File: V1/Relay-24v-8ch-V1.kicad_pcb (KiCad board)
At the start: 2 copper layers, 108 x 67.8 mm, 49 parts, among them J1 Conn_01x09, J2 OUT1, J3 OUT2, J4 OUT3, J5 OUT4, J6 OUT5, J7 OUT6, J8 OUT7, J9 OUT8, K1 G5PZ-1A, K2 G5PZ-1A, K3 G5PZ-1A, K4 G5PZ-1A, K5 G5PZ-1A, K6 G5PZ-1A, K7 G5PZ-1A, K8 G5PZ-1A

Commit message: Adjustments for fabrication
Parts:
- D11, D12, D15, D16, D3, D4, D7, D8: value BLUE/0603 -> GREEN/0603
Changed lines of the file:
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@@
     (property "Case" "0603")
     (property "JLCPCB BOM" "1")
-    (property "LCSC Part #" "C72041")
+    (property "LCSC Part #" "C72043")
     (property "Mfr" "Everlight")
-    (property "Mfr PN" "19-217/BHC-ZL1M2RY/3T")
+    (property "Mfr PN" "19-217/GHC-YR1S2/3T")
     (property "Sheetfile" "Relay-24v-8ch-V1.kicad_sch")
     (property "Sheetname" "")
     (property "Technology" "")
     (property "Vendor" "JLCPCB")
-    (property "Vendor PN" "C72041")
+    (property "Vendor PN" "C72043")
     (property "ki_description" "Light emitting diode")
     (property "ki_keywords" "LED diode")
@@
         (effects (font (size 1 1) (thickness 0.15)))
     )
-    (fp_text value "BLUE/0603" (at 0 1.43) (layer "F.Fab")
+    (fp_text value "GREEN/0603" (at 0 1.43) (layer "F.Fab")
         (effects (font (size 1 1) (thickness 0.15)))
     )
@@
     (property "Case" "0603")
     (property "JLCPCB BOM" "1")
-    (property "LCSC Part #" "C72041")
+    (property "LCSC Part #" "C72043")
     (property "Mfr" "Everlight")
-    (property "Mfr PN" "19-217/BHC-ZL1M2RY/3T")
+    (property "Mfr PN" "19-217/GHC-YR1S2/3T")
     (property "Sheetfile" "Relay-24v-8ch-V1.kicad_sch")
     (property "Sheetname" "")
     (property "Technology" "")
     (property "Vendor" "JLCPCB")
-    (property "Vendor PN" "C72041")
+    (property "Vendor PN" "C72043")
     (property "ki_description" "Light emitting diode")
     (property "ki_keywords" "LED diode")
@@
         (effects (font (size 1 1) (thickness 0.15)))
     )
-    (fp_text value "BLUE/0603" (at 0 1.43) (layer "F.Fab")
+    (fp_text value "GREEN/0603" (at 0 1.43) (layer "F.Fab")
         (effects (font (size 1 1) (thickness 0.15)))
     )
@@
     (property "Case" "0603")
     (property "JLCPCB BOM" "1")
-    (property "LCSC Part #" "C72041")
+    (property "LCSC Part #" "C72043")
     (property "Mfr" "Everlight")
-    (property "Mfr PN" "19-217/BHC-ZL1M2RY/3T")
+    (property "Mfr PN" "19-217/GHC-YR1S2/3T")
     (property "Sheetfile" "Relay-24v-8ch-V1.kicad_sch")
     (property "Sheetname" "")
     (property "Technology" "")
     (property "Vendor" "JLCPCB")
-    (property "Vendor PN" "C72041")
+    (property "Vendor PN" "C72043")
     (property "ki_description" "Light emitting diode")
     (property "ki_keywords" "LED diode")
@@
         (effects (font (size 1 1) (thickness 0.15)))
     )
-    (fp_text value "BLUE/0603" (at 0 1.43) (layer "F.Fab")
+    (fp_text value "GREEN/0603" (at 0 1.43) (layer "F.Fab")
         (effects (font (size 1 1) (thickness 0.15)))
     )
@@
     (property "Case" "0603")
     (property "JLCPCB BOM" "1")
-    (property "LCSC Part #" "C72041")
+    (property "LCSC Part #" "C72043")
     (property "Mfr" "Everlight")
-    (property "Mfr PN" "19-217/BHC-ZL1M2RY/3T")
+    (property "Mfr PN" "19-217/GHC-YR1S2/3T")
     (property "Sheetfile" "Relay-24v-8ch-V1.kicad_sch")
     (property "Sheetname" "")
     (property "Technology" "")
     (property "Vendor" "JLCPCB")
-    (property "Vendor PN" "C72041")
+    (property "Vendor PN" "C72043")
     (property "ki_description" "Light emitting diode")
     (property "ki_keywords" "LED diode")
@@
         (effects (font (size 1 1) (thickness 0.15)))
     )
-    (fp_text value "BLUE/0603" (at 0 1.43) (layer "F.Fab")
+    (fp_text value "GREEN/0603" (at 0 1.43) (layer "F.Fab")
         (effects (font (size 1 1) (thickness 0.15)))
     )
@@
     (property "Case" "0603")
     (property "JLCPCB BOM" "1")
-    (property "LCSC Part #" "C72041")
+    (property "LCSC Part #" "C72043")
     (property "Mfr" "Everlight")
-    (property "Mfr PN" "19-217/BHC-ZL1M2RY/3T")
+    (property "Mfr PN" "19-217/GHC-YR1S2/3T")
     (property "Sheetfile" "Relay-24v-8ch-V1.kicad_sch")
     (property "Sheetname" "")
     (property "Technology" "")
     (property "Vendor" "JLCPCB")
-    (property "Vendor PN" "C72041")
+    (property "Vendor PN" "C72043")
     (property "ki_description" "Light emitting diode")
     (property "ki_keywords" "LED diode")
@@
         (effects (font (size 1 1) (thickness 0.15)))
     )
-    (fp_text value "BLUE/0603" (at 0 1.43) (layer "F.Fab")
+    (fp_text value "GREEN/0603" (at 0 1.43) (layer "F.Fab")
         (effects (font (size 1 1) (thickness 0.15)))
     )
@@
     (property "Case" "0603")
     (property "JLCPCB BOM" "1")
-    (property "LCSC Part #" "C72041")
+    (property "LCSC Part #" "C72043")
     (property "Mfr" "Everlight")
-    (property "Mfr PN" "19-217/BHC-ZL1M2RY/3T")
+    (property "Mfr PN" "19-217/GHC-YR1S2/3T")
     (property "Sheetfile" "Relay-24v-8ch-V1.kicad_sch")
     (property "Sheetname" "")
     (property "Technology" "")
     (property "Vendor" "JLCPCB")
-    (property "Vendor PN" "C72041")
+    (property "Vendor PN" "C72043")
     (property "ki_description" "Light emitting diode")
     (property "ki_keywords" "LED diode")
@@
         (effects (font (size 1 1) (thickness 0.15)))
     )
-    (fp_text value "BLUE/0603" (at 0 1.43) (layer "F.Fab")
+    (fp_text value "GREEN/0603" (at 0 1.43) (layer "F.Fab")
         (effects (font (size 1 1) (thickness 0.15)))
     )
@@
     (property "Case" "0603")
     (property "JLCPCB BOM" "1")
-    (property "LCSC Part #" "C72041")
+    (property "LCSC Part #" "C72043")
     (property "Mfr" "Everlight")
-    (property "Mfr PN" "19-217/BHC-ZL1M2RY/3T")
+    (property "Mfr PN" "19-217/GHC-YR1S2/3T")
     (property "Sheetfile" "Relay-24v-8ch-V1.kicad_sch")
     (property "Sheetname" "")
     (property "Technology" "")
     (property "Vendor" "JLCPCB")
-    (property "Vendor PN" "C72041")
+    (property "Vendor PN" "C72043")
     (property "ki_description" "Light emitting diode")
     (property "ki_keywords" "LED diode")
@@
         (effects (font (size 1 1) (thickness 0.15)))
     )
-    (fp_text value "BLUE/0603" (at 0 1.43) (layer "F.Fab")
+    (fp_text value "GREEN/0603" (at 0 1.43) (layer "F.Fab")
         (effects (font (size 1 1) (thickness 0.15)))
     )
@@
     (property "Case" "0603")
     (property "JLCPCB BOM" "1")
-    (property "LCSC Part #" "C72041")
+    (property "LCSC Part #" "C72043")
     (property "Mfr" "Everlight")
-    (property "Mfr PN" "19-217/BHC-ZL1M2RY/3T")
+    (property "Mfr PN" "19-217/GHC-YR1S2/3T")
     (property "Sheetfile" "Relay-24v-8ch-V1.kicad_sch")
     (property "Sheetname" "")
     (property "Technology" "")
     (property "Vendor" "JLCPCB")
-    (property "Vendor PN" "C72041")
+    (property "Vendor PN" "C72043")
     (property "ki_description" "Light emitting diode")
     (property "ki_keywords" "LED diode")
@@
         (effects (font (size 1 1) (thickness 0.15)))
     )
-    (fp_text value "BLUE/0603" (at 0 1.43) (layer "F.Fab")
+    (fp_text value "GREEN/0603" (at 0 1.43) (layer "F.Fab")
         (effects (font (size 1 1) (thickness 0.15)))
     )

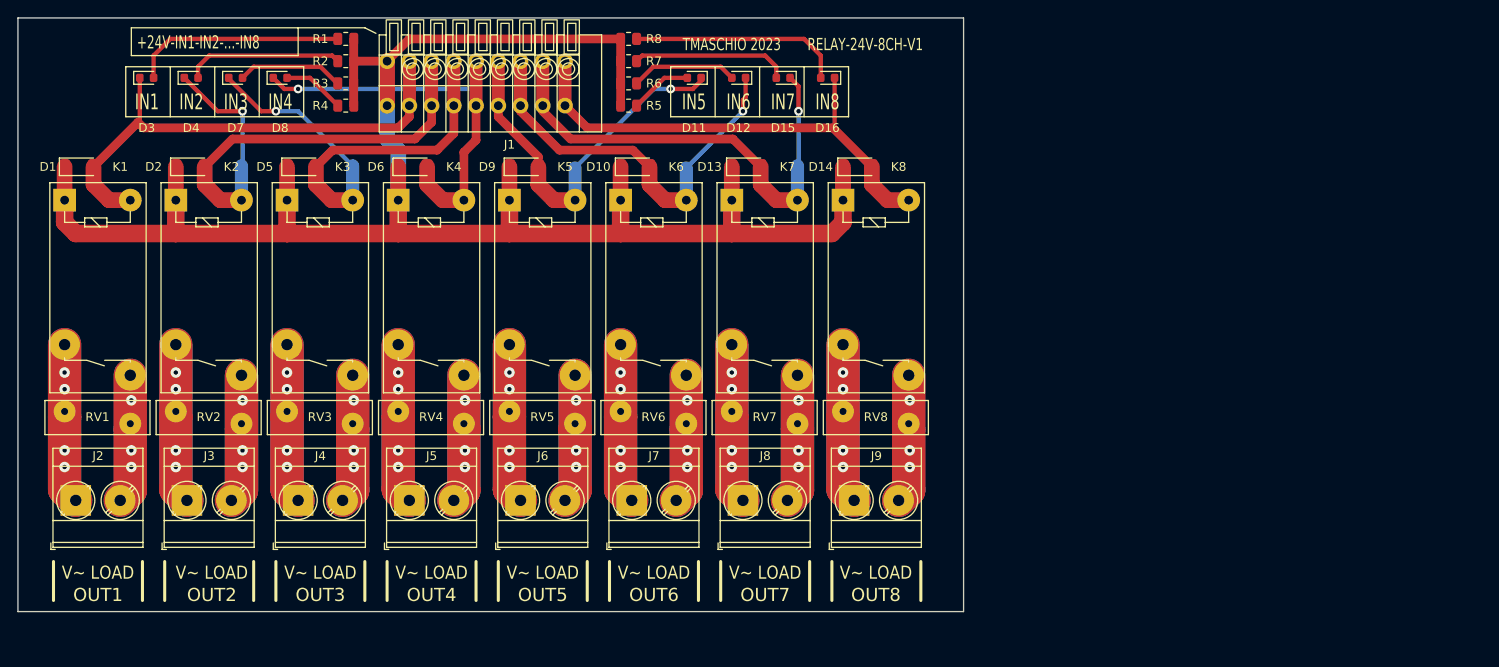
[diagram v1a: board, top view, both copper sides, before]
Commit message: Cleanup
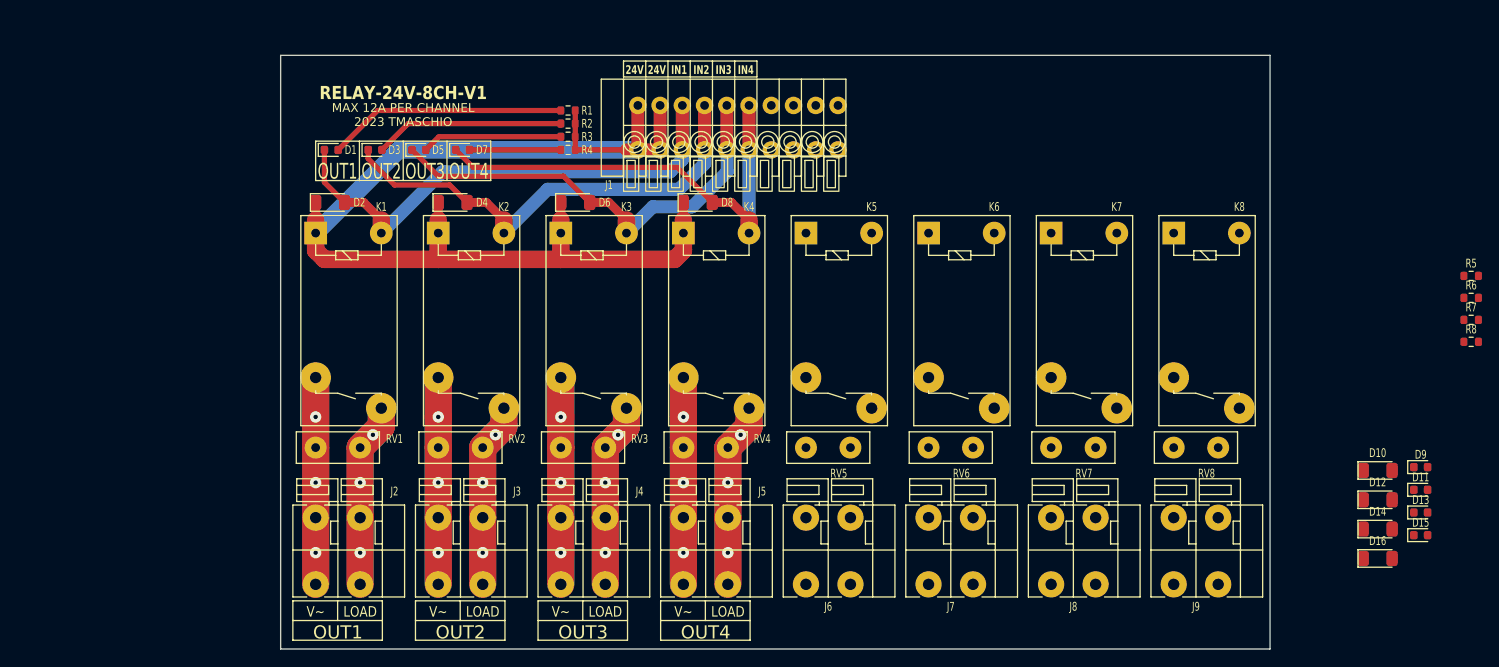
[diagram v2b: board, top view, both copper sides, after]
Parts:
- D1: renamed from D3; value GREEN/0603 -> GREEN
- D10, D14: value 1N4148/SOD-123 -> 1N4148
- D11, D15: value GREEN/0603 -> GREEN
- D12, D16: value GREEN/0603 -> 1N4148; footprint Tales:LED_0603_1608Metric -> Tales:D_SOD-123
- D13, D9: value 1N4148/SOD-123 -> GREEN; footprint Tales:D_SOD-123 -> Tales:LED_0603_1608Metric
- D2: renamed from D1; value 1N4148/SOD-123 -> 1N4148
- D3: renamed from D4; value GREEN/0603 -> GREEN
- D4: renamed from D2; value 1N4148/SOD-123 -> 1N4148
- D5: renamed from D7; value GREEN/0603 -> GREEN
- D6: renamed from D5; value 1N4148/SOD-123 -> 1N4148
- D7: renamed from D8; value GREEN/0603 -> GREEN
- D8: renamed from D6; value 1N4148/SOD-123 -> 1N4148
- J1: value Conn_01x09 -> DB141V-2.54-10P; footprint Tales:TerminalBlock_DG141V-2.54-9P_1x09_P2.54mm_Vertical -> Tales:TerminalBlock_Dibo_DB141V-2.54-10P_1x10_P2.54mm_Vertical
- J2: value OUT1 -> DB142V-5.08-2P; footprint Tales:TerminalBlock_Phoenix_MKDS-3-2-5.08_1x02_P5.08mm_Horizontal -> Tales:TerminalBlock_Dibo_DB142V-5.08-2P_1x02_P5.08mm_Vertical
- J3: value OUT2 -> DB142V-5.08-2P; footprint Tales:TerminalBlock_Phoenix_MKDS-3-2-5.08_1x02_P5.08mm_Horizontal -> Tales:TerminalBlock_Dibo_DB142V-5.08-2P_1x02_P5.08mm_Vertical
- J4: value OUT3 -> DB142V-5.08-2P; footprint Tales:TerminalBlock_Phoenix_MKDS-3-2-5.08_1x02_P5.08mm_Horizontal -> Tales:TerminalBlock_Dibo_DB142V-5.08-2P_1x02_P5.08mm_Vertical
- J5: value OUT4 -> DB142V-5.08-2P; footprint Tales:TerminalBlock_Phoenix_MKDS-3-2-5.08_1x02_P5.08mm_Horizontal -> Tales:TerminalBlock_Dibo_DB142V-5.08-2P_1x02_P5.08mm_Vertical
- J6: value OUT5 -> DB142V-5.08-2P; footprint Tales:TerminalBlock_Phoenix_MKDS-3-2-5.08_1x02_P5.08mm_Horizontal -> Tales:TerminalBlock_Dibo_DB142V-5.08-2P_1x02_P5.08mm_Vertical
- J7: value OUT6 -> DB142V-5.08-2P; footprint Tales:TerminalBlock_Phoenix_MKDS-3-2-5.08_1x02_P5.08mm_Horizontal -> Tales:TerminalBlock_Dibo_DB142V-5.08-2P_1x02_P5.08mm_Vertical
- J8: value OUT7 -> DB142V-5.08-2P; footprint Tales:TerminalBlock_Phoenix_MKDS-3-2-5.08_1x02_P5.08mm_Horizontal -> Tales:TerminalBlock_Dibo_DB142V-5.08-2P_1x02_P5.08mm_Vertical
- J9: value OUT8 -> DB142V-5.08-2P; footprint Tales:TerminalBlock_Phoenix_MKDS-3-2-5.08_1x02_P5.08mm_Horizontal -> Tales:TerminalBlock_Dibo_DB142V-5.08-2P_1x02_P5.08mm_Vertical
- K1, K2, K3, K4, K5, K6, K7, K8: footprint Tales:Relay_SPST_Omron-G5PZ-1A -> Tales:Relay_SPST_Omron_G5PZ-1A
- R1, R2, R3, R4, R5, R6, R7, R8: value 4k7/0,125W/0805 -> 5k6/100mW; footprint Tales:R_0805_2012Metric -> Tales:R_0603_1608Metric
- RV1, RV2, RV3, RV4, RV5, RV6, RV7, RV8: value 250VAC -> 275VAC; footprint Tales:RV_Disc_D12mm_W3.9mm_P7.5mm -> Tales:RV_Disc_D9.50mm_W3.6mm_P5.08mm
- moved D9 108.0 mm to (255.2, 109.2)
- moved R8 102.3 mm to (261.0, 94.9)
- moved R7 100.7 mm to (261.0, 92.4)
- moved R6 99.3 mm to (261.0, 89.9)
- moved R5 98.2 mm to (261.0, 87.4)
- moved D11 95.4 mm to (255.2, 111.8), turned to 0 degrees
- moved D10 91.6 mm to (250.3, 109.6)
- moved D15 89.6 mm to (255.2, 117.0), turned to 0 degrees
- moved D12 87.5 mm to (250.3, 113.0), turned to 0 degrees
- moved D13 86.6 mm to (255.2, 114.4)
- moved D16 83.4 mm to (250.3, 119.7), turned to 0 degrees
- moved D14 72.4 mm to (250.3, 116.3)
- moved RV8 38.0 mm to (227.0, 107.0)
- moved K8 38.0 mm to (227.0, 82.5)
- moved J9 37.7 mm to (227.0, 122.6)
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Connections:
- D12 pad 1: Net-(D10-A) -> +24V
- D12 pad 2: Net-(D12-A) -> Net-(D11-K)
- D13 pad 1: +24V -> Net-(D13-K)
- D14 pad 2: Net-(D14-A) -> Net-(D13-K)
- D15 pad 1: Net-(D13-A) -> Net-(D15-K)
- D16 pad 1: Net-(D14-A) -> +24V
- D16 pad 2: Net-(D16-A) -> Net-(D15-K)
- D9 pad 1: +24V -> Net-(D10-A)
- D9 pad 2: Net-(D11-K) -> Net-(D9-A)
- J1 pad 1: Net-(D14-A) -> Net-(D15-K)
- J1 pad 2: Net-(D13-A) -> Net-(D13-K)
- J1 pad 3: Net-(D10-A) -> Net-(D11-K)
- J1 pad 4: Net-(D11-K) -> Net-(D10-A)
- K5 pad 4: Net-(D11-K) -> Net-(D10-A)
- K6 pad 4: Net-(D10-A) -> Net-(D11-K)
- K7 pad 4: Net-(D13-A) -> Net-(D13-K)
- K8 pad 4: Net-(D14-A) -> Net-(D15-K)
- R5 pad 2: Net-(D11-A) -> Net-(D9-A)
- R6 pad 2: Net-(D12-A) -> Net-(D11-A)
- R7 pad 2: Net-(D15-A) -> Net-(D13-A)
- R8 pad 2: Net-(D16-A) -> Net-(D15-A)
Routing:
- net +24V: track 211.5 -> 131.9 mm
- net Net-(D14-A): track 55.8 -> 0.00 mm
- net Net-(D13-A): track 54.6 -> 0.00 mm, vias 1 -> 0
- net Net-(D10-A): track 46.8 -> 0.00 mm, vias 1 -> 0
- net Net-(D11-K): track 43.5 -> 0.00 mm, vias 1 -> 0
- net Net-(J9-Pin_1): track 36.6 -> 0.00 mm, vias 4 -> 0
- net Net-(J8-Pin_1): track 36.6 -> 0.00 mm, vias 4 -> 0
- net Net-(J6-Pin_1): track 36.6 -> 0.00 mm, vias 4 -> 0
- net Net-(J7-Pin_1): track 36.6 -> 0.00 mm, vias 4 -> 0
- net Net-(J8-Pin_2): track 29.5 -> 0.00 mm, vias 3 -> 0
- net Net-(J7-Pin_2): track 29.5 -> 0.00 mm, vias 3 -> 0
- net Net-(J6-Pin_2): track 29.5 -> 0.00 mm, vias 3 -> 0
- net Net-(J9-Pin_2): track 29.5 -> 0.00 mm, vias 3 -> 0
- net Net-(D16-A): track 24.4 -> 0.00 mm
- net Net-(D15-A): track 18.0 -> 0.00 mm
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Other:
- board size 108 x 67.8 mm -> 113 x 67.8 mm
- board text added: "24V"
- board text added: "CORRENTE MÁXIMA POR CANAL CONSIDERAÇÕES: - ESPESSURA COBRE 0,035mm, TRILHAS EM AMBOS LAYERS, EQUIVALE 0,070mm - deltaT NA TRILHA 20ºC - LARGURA DE TRILHA NECESSÁRIA PARA 12A = 3,03726mm TRILHAS DESENHADAS EM AMBOS OS LAYERS COM 3,1mm DE LARGURA"
- board text added: "LOAD"
- board text added: "MAX 12A PER CHANNEL 2023 TMASCHIO"
- board text added: "SUPORTES PCI METALTEX SP7 1x pé macho 9 mm 1x pé fêmea 9 mm 1x espaçador 30 mm 1x espaçador 10 mm Comprimento total 58 mm Largura da placa 67,8 mm"
- board text added: "V~"
- board text removed: "+24V-IN1-IN2-...-IN8"
- board text removed: "IN5"
- board text removed: "IN6"
- board text removed: "IN7"
- board text removed: "IN8"
- board text removed: "OUT5"
- board text removed: "OUT6"
- board text removed: "OUT7"
- board text removed: "OUT8"
- board text removed: "SUPORTES PCI METALTEX SP7 1x pé macho 9 mm 1x pé fêmea 9 mm 2x espaçadores 45 mm Comprimento total 108 mm Largura da placa 67,8 mm"
- board text removed: "TMASCHIO 2023"
- board text removed: "V~ LOAD"
